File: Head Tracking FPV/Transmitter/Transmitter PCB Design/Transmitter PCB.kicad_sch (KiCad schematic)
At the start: 6 parts, among them J1 Conn_01x02_Pin, J2 Conn_01x03_Pin, U1 ESP32-DEVKIT-V1, U2 OC09600

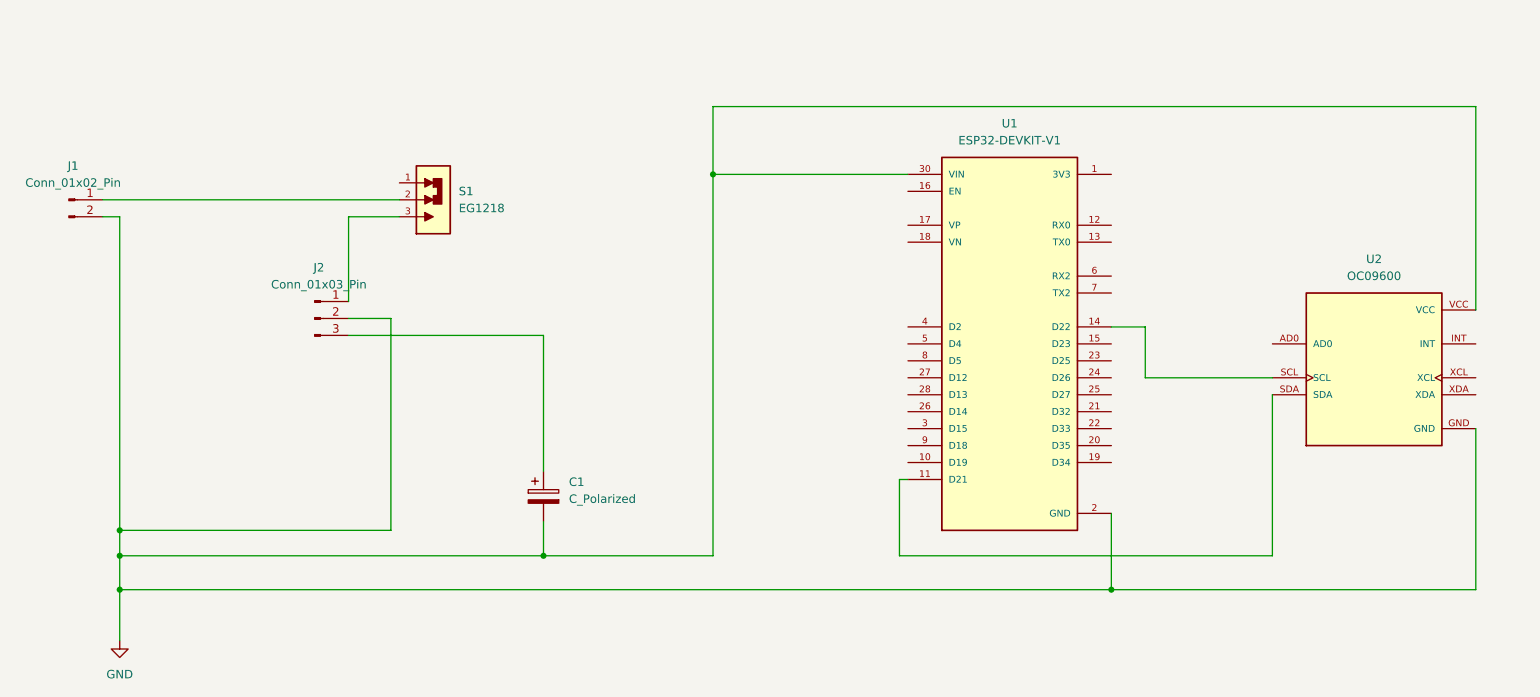
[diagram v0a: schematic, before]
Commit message: Finished Transmitter PCB
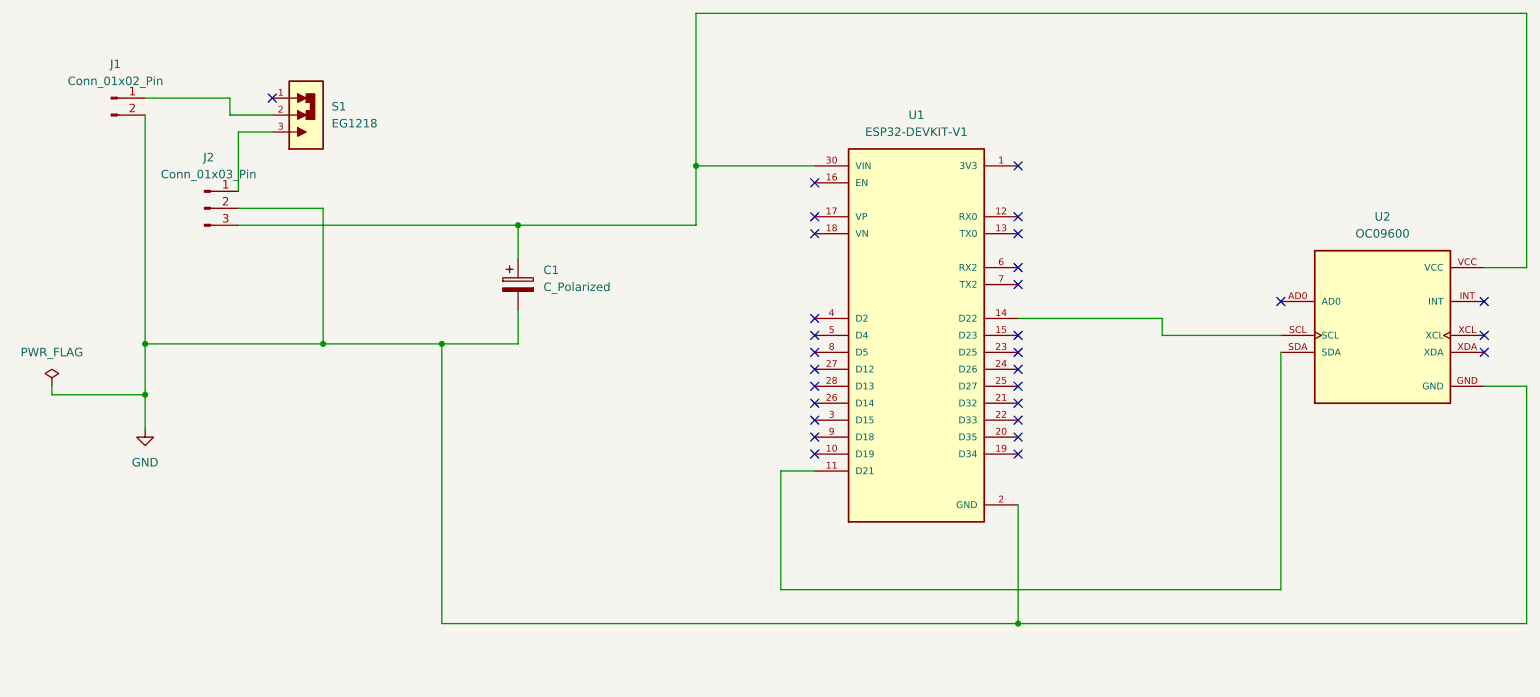
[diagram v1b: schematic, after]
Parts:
- C1: footprint (none) -> Capacitor_THT:CP_Radial_D5.0mm_P2.00mm
- J1: footprint (none) -> Connector_JST:JST_PH_S2B-PH-K_1x02_P2.00mm_Horizontal
- J2: footprint (none) -> Connector_PinHeader_2.54mm:PinHeader_1x03_P2.54mm_Vertical
- S1: footprint EG1218:SW_EG1218 -> Slide Switch (EG1218):SW_EG1218
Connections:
- net GND: no longer U1.30 (VIN), U2.VCC
- net at C1.1, J2.3 (Pin_3): now also U1.30 (VIN), U2.VCC
- no-connect marks 0 -> 30
